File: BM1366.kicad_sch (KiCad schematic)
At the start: 1 part, among them U1 TPS4030x

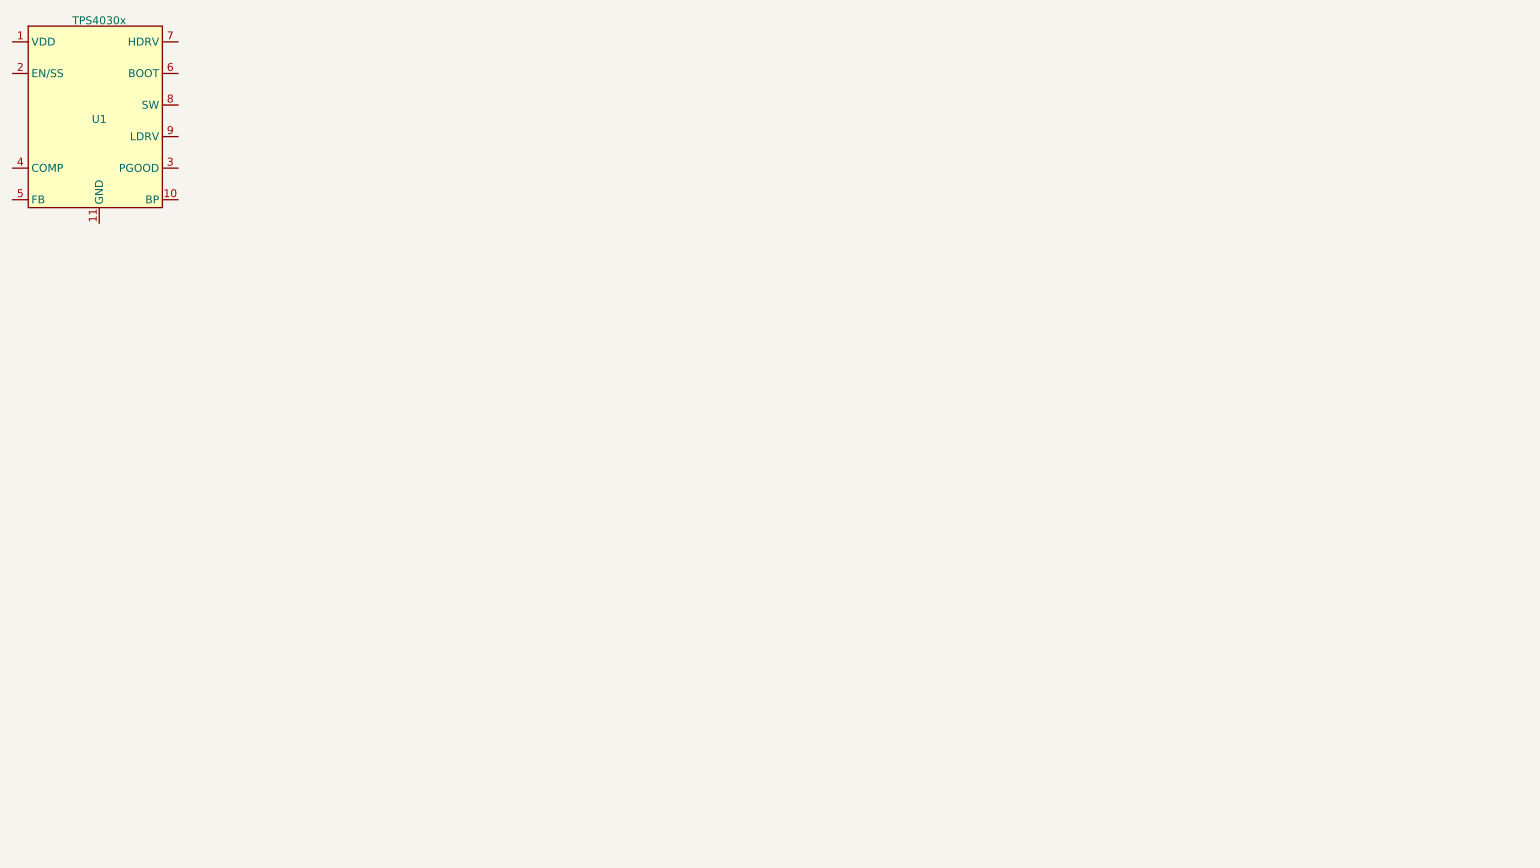
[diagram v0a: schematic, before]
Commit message: did some stuffs
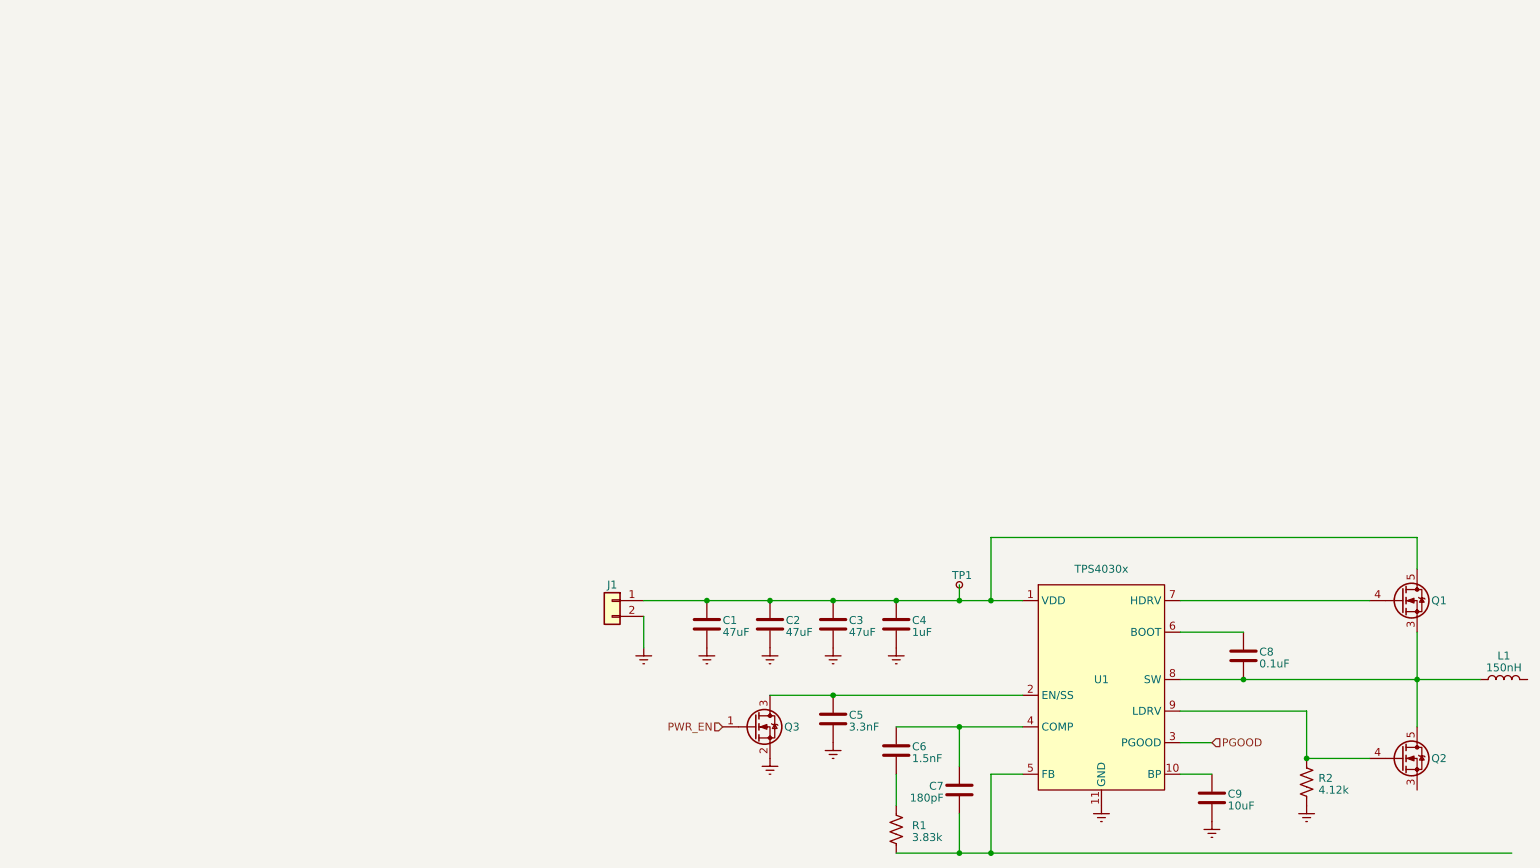
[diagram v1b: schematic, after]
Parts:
- added C1, C2, C3: 47uF, Capacitor_SMD:C_1210_3225Metric, symbol Device:C
- added C4: 1uF, Capacitor_SMD:C_0805_2012Metric, symbol Device:C
- added C5: 3.3nF, Capacitor_SMD:C_0402_1005Metric, symbol Device:C
- added C6: 1.5nF, Capacitor_SMD:C_0805_2012Metric, symbol Device:C
- added C7: 180pF, Capacitor_SMD:C_0805_2012Metric, symbol Device:C
- added C8: 0.1uF, Capacitor_SMD:C_0402_1005Metric, symbol Device:C
- added C9: 10uF, Capacitor_SMD:C_0805_2012Metric, symbol Device:C
- added J1: Conn_01x02, symbol Connector_Generic:Conn_01x02
- added L1: 150nH, Library:FP1005R1-R15-R, symbol Device:L
- added Q1, Q2: CSD17311Q5, Library:CSD17576Q5B, symbol bitaxe:Q_NMOS_CSD17311Q5_1
- added Q3: 2N7002K, Package_TO_SOT_SMD:SOT-323_SC-70, symbol Transistor_FET:2N7002K
- added R1: 3.83k, Resistor_SMD:R_0402_1005Metric, symbol Device:R_US
- added R2: 4.12k, Resistor_SMD:R_0402_1005Metric, symbol Device:R_US
- added TP1: TestPoint_Small, symbol Connector:TestPoint_Small
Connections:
- net at U1.1 (VDD): now also C1.1, C2.1, C3.1, C4.1, J1.1 (Pin_1), Q1.5 (D), TP1.1
- net at U1.10 (BP): now also C9.1
- net Earth: now reaches U1.11 (GND)
- net Earth: now also C1.2, C2.2, C3.2, C4.2, C5.1, C9.2, J1.2 (Pin_2), Q3.2 (S), R2.2
- net at U1.2 (EN/SS): now also C5.2, Q3.3 (D)
- net PGOOD: now reaches U1.3 (PGOOD)
- net at U1.4 (COMP): now also C6.1, C7.2
- net at U1.5 (FB): now also C7.1, R1.2
- net at U1.6 (BOOT): now also C8.1
- net at U1.7 (HDRV): now also Q1.4 (G)
- net at U1.8 (SW): now also C8.2, L1.1, Q1.1, Q1.2, Q1.3 (S), Q2.5 (D)
- net at U1.9 (LDRV): now also Q2.4 (G), R2.1
- new net: C6.2, R1.1
- new net: Q2.1, Q2.2, Q2.3 (S)
- new net PWR_EN: Q3.1 (G)
